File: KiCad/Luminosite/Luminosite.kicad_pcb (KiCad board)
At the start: 2 copper layers, 43.8 x 29.6 mm, 33 parts, among them J1 Conn_01x03_Pin, J2 Conn_01x02_Pin, J3 Conn_01x02_Pin, K1 TQ2-L2-5V, Q3 BC547C, Q4 BC547C, U1 MCP6022, U2 TL431D, U3 MCP6022, U4 ESP32-C3_SUPERMINI_TH

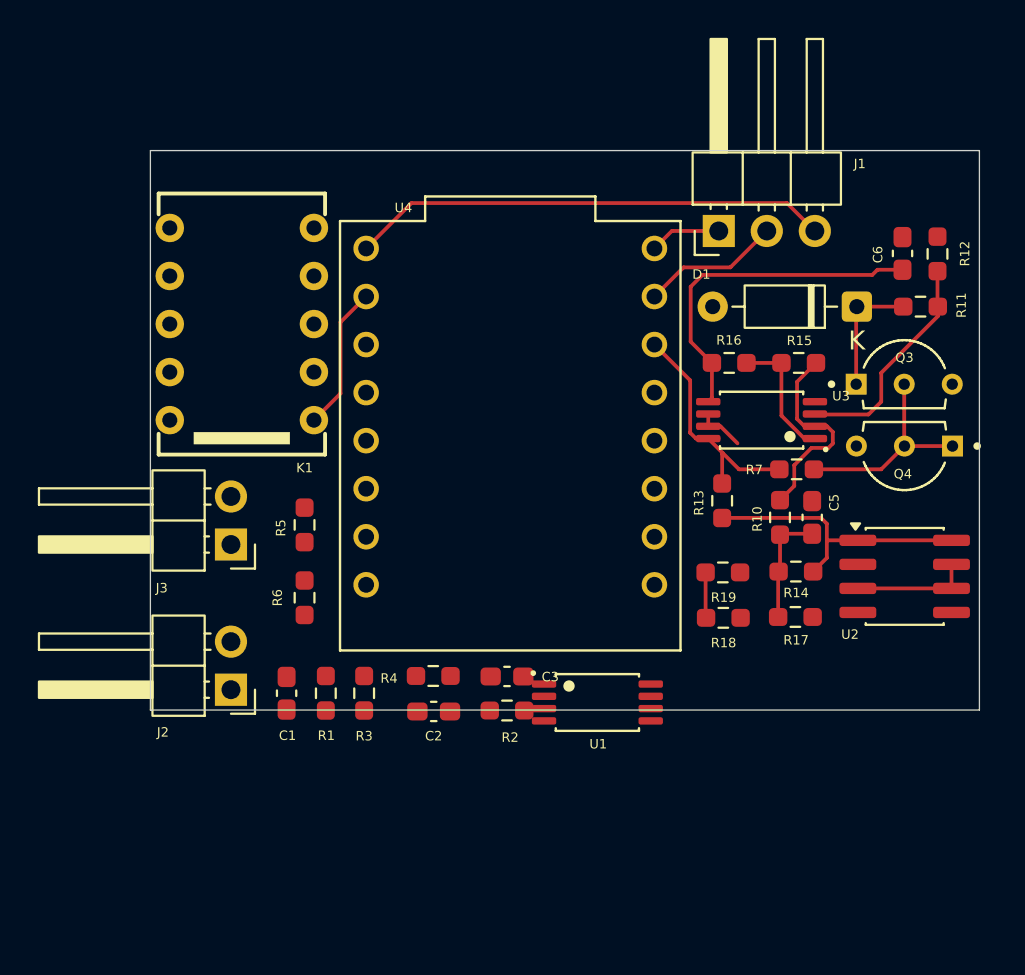
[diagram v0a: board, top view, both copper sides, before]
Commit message: PCB Terminé
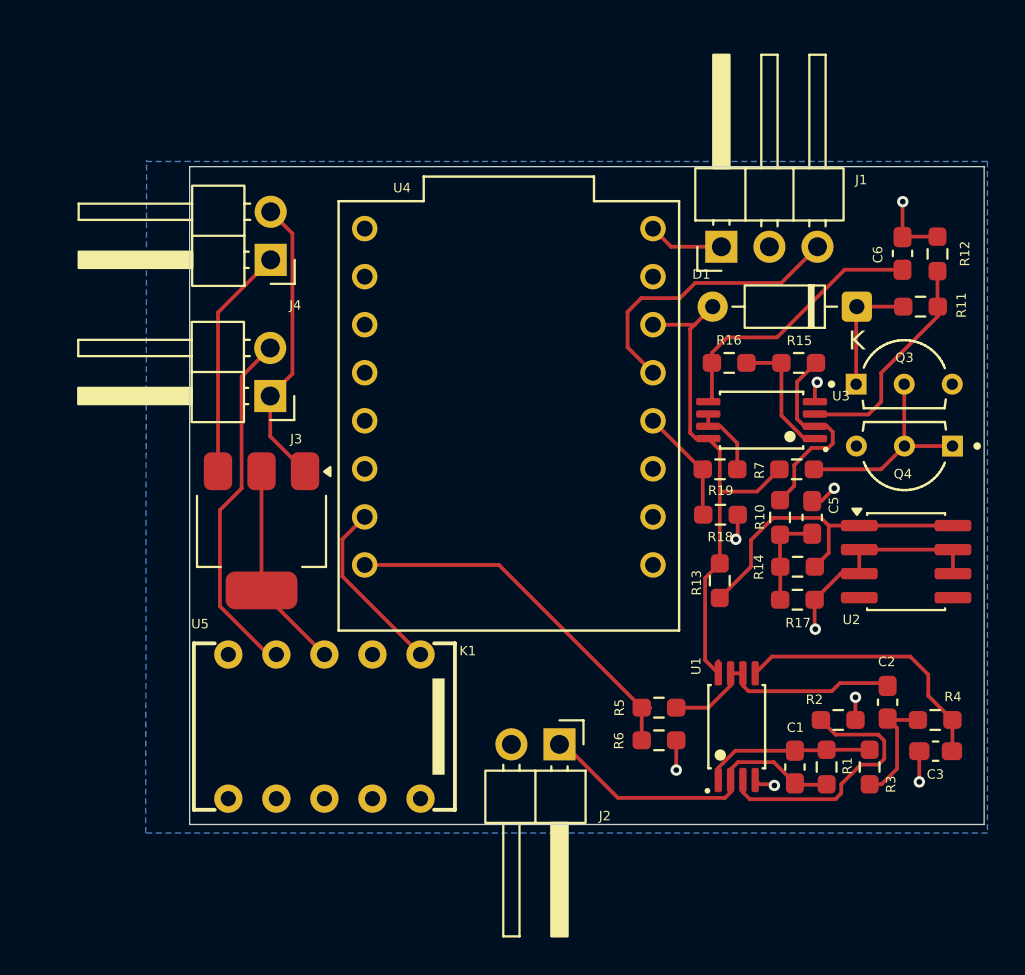
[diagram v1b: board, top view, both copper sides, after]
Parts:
- added J4: Conn_01x02_Pin, Connector_PinHeader_2.54mm:PinHeader_1x02_P2.54mm_Horizontal, F.Cu at (123.3, 73.5)
- added U5: AMS1117-5.0, Package_TO_SOT_SMD:SOT-223-3_TabPin2, F.Cu at (122.8, 87.8)
- moved C1 27.2 mm to (151.0, 100.3)
- moved R3 27.0 mm to (155.0, 100.3)
- moved R1 26.8 mm to (152.7, 100.3)
- moved R4 26.6 mm to (158.5, 97.8)
- moved C2 24.0 mm to (155.9, 96.9), turned to 90 degrees
- moved C3 23.0 mm to (158.5, 99.5), turned to 0 degrees
- moved K1 21.7 mm to (126.2, 98.2), turned to 180 degrees
- moved R5 21.1 mm to (143.9, 97.2), turned to 0 degrees
- moved R6 20.2 mm to (143.9, 98.9), turned to 180 degrees
- moved J2 17.6 mm to (138.6, 99.1), turned to -90 degrees
- moved R2 17.5 mm to (153.3, 97.8), turned to 0 degrees
- moved J3 8.12 mm to (123.3, 80.7)
- moved U1 7.48 mm to (148.0, 98.2), turned to 90 degrees
- moved R19 5.45 mm to (147.1, 84.6)
- moved R18 5.45 mm to (147.1, 87.0)
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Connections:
- J3 pad 1: GND -> Net-(J3-Pin_1)
- K1 pad 3: +5V -> Net-(U5-VO)
- U4 pad 10: Luminosité_OUT -> unconnected-(U4-GPIO10-Pad10)
- U4 pad 20: unconnected-(U4-GPIO20-Pad20) -> Pompe_OUT
- U4 pad 21: unconnected-(U4-GPIO21-Pad21) -> Luminosité_OUT
- U4 pad 4: unconnected-(U4-GPIO4-Pad4) -> Humidite_OUT
- U4 pad 5: Humidite_OUT -> unconnected-(U4-GPIO5-Pad5)
- U4 pad 6: Pompe_OUT -> unconnected-(U4-GPIO6-Pad6)
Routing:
- net Luminosité_OUT: track 0.00 -> 19.9 mm
- net Net-(J3-Pin_2): track 0.00 -> 18.8 mm
- net Net-(J2-Pin_1): track 0.00 -> 17.3 mm
- net +3.3V: track 13.1 -> 29.9 mm
- net Net-(J3-Pin_1): track 0.00 -> 15.4 mm
- net Net-(U1B-+): track 0.00 -> 14.5 mm
- net Net-(U1A-+): track 0.00 -> 14.2 mm
- net Net-(U1B--): track 0.00 -> 13.3 mm
- net Net-(J4-Pin_1): track 0.00 -> 12.3 mm
- net GND: track 13.6 -> 25.1 mm, vias 0 -> 9
- net Net-(U5-VO): track 0.00 -> 11.1 mm
- net Humidite_OUT: track 25.3 -> 15.2 mm
- net Net-(C1-Pad2): track 0.00 -> 9.17 mm
- net Net-(C2-Pad1): track 0.00 -> 6.28 mm
- net Température_OUT: track 2.41 -> 6.10 mm
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- added copper zone on B.Cu, net GND
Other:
- board size 43.8 x 29.6 mm -> 42 x 34.8 mm
